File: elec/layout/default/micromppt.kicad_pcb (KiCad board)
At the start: 2 copper layers, 25.9 x 15.3 mm, 16 parts

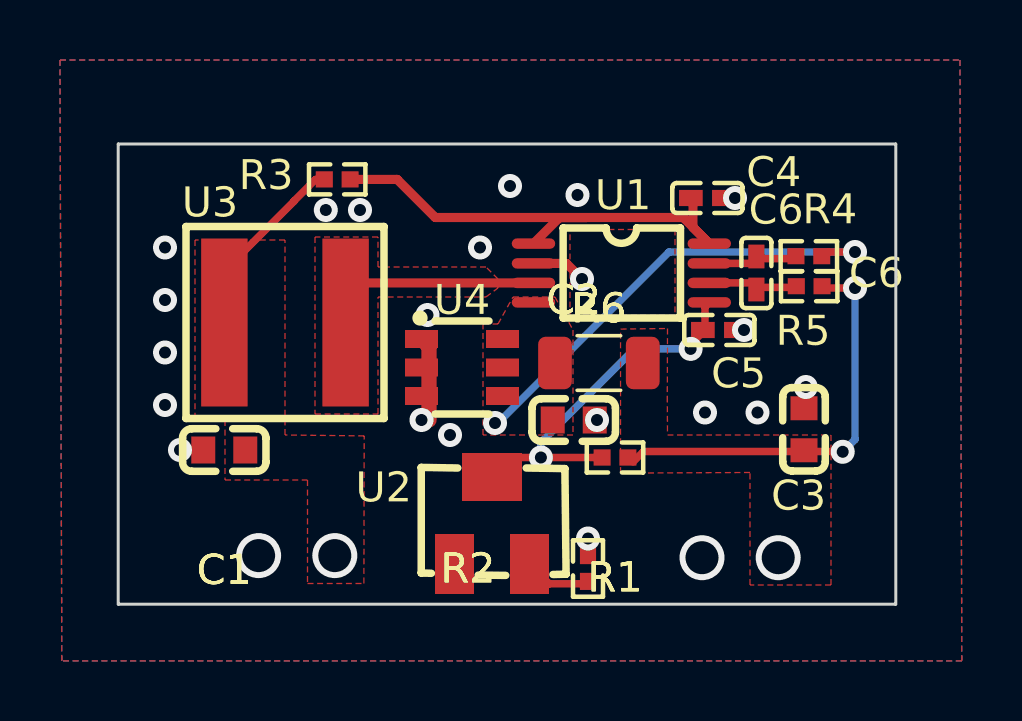
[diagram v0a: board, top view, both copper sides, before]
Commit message: fixed :woozy:
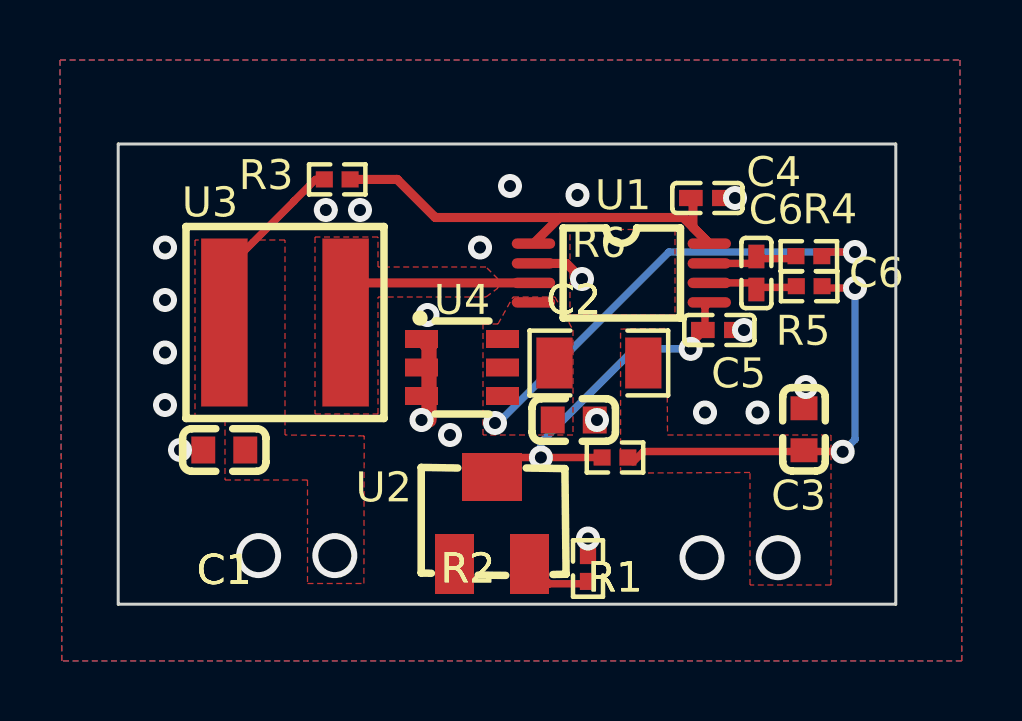
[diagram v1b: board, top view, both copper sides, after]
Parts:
- C5: value 1nF ±10% 50V X7R -> 1nF ±20% 50V X7R
- R6: footprint lib:R1206 -> atopile:R1206-bdb864
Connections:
- C1 pad 1: hv-1 -> hv
- C3 pad 1: hv -> hv-1
- R1 pad 1: hv -> hv-1
- R2 pad 1: p3 -> net
- R3 pad 1: hv-1 -> hv
- R5 pad 2: hv -> hv-1
- R6 pad 2: hv -> hv-1
- U2 pad 1: net -> VR2-net
- U2 pad 3: p3 -> net
- U3 pad 1: hv-1 -> hv
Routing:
- net hv-1: track 8.72 -> 13.9 mm, vias 1 -> 3
- net hv: track 13.9 -> 8.72 mm, vias 3 -> 1
- net p3: track 2.22 -> 0.00 mm
- net net: track 0.00 -> 2.22 mm
